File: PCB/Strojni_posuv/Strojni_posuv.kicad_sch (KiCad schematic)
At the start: 58 parts, among them J1 Conn_01x20_Pin, J15 Conn_01x06_Socket, J7 Button_maxL, J9 Button_maxR, SW1 SW_SPDT_MSM, SW2 SW_DPST_x2, SW3 SW_DPST_x2, SW4 SW_SPDT, SW5 RotaryEncoder_Switch, U1 STM32F103RBTx, Y1 16MHz

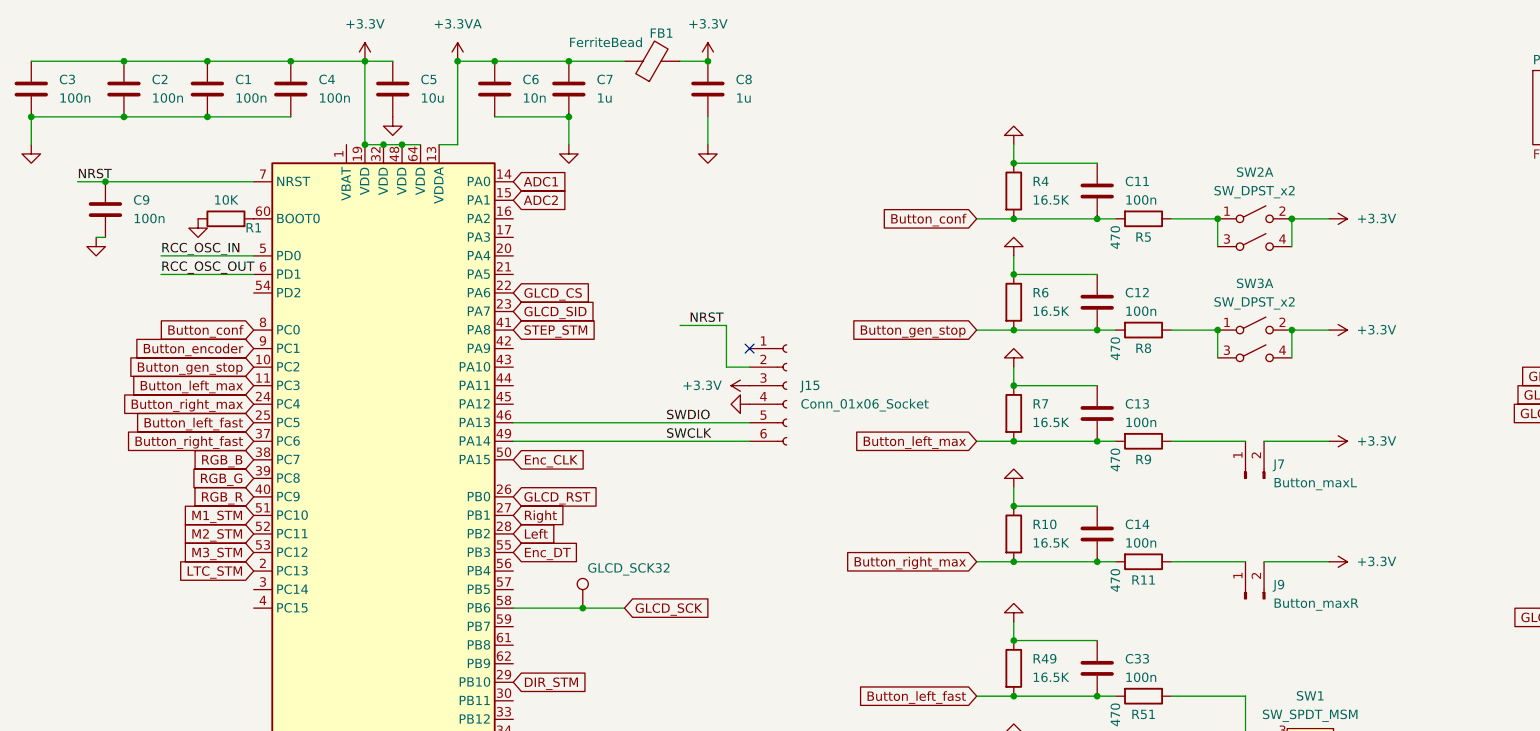
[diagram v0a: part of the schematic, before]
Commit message: Resolving problems from list
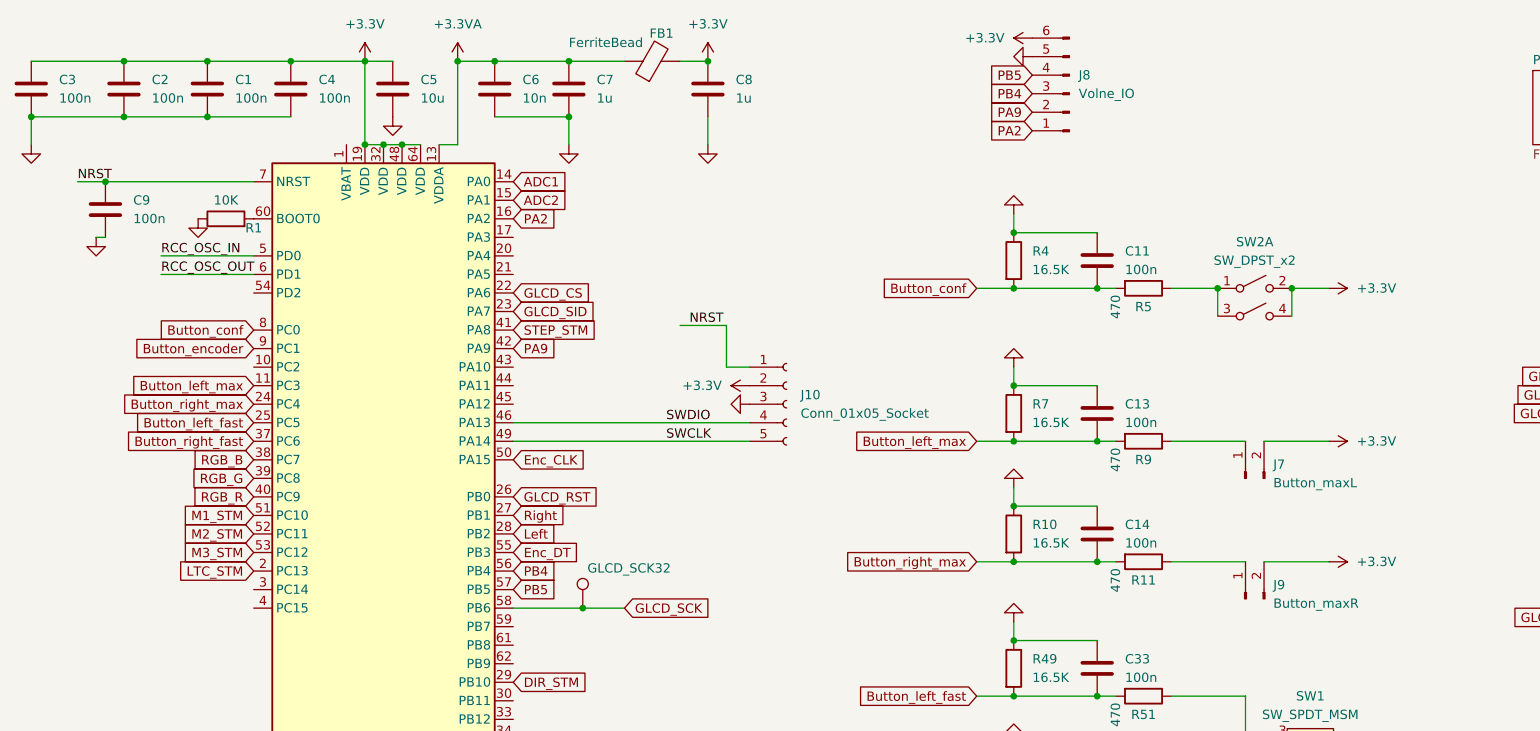
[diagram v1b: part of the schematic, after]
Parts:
- removed C12: 100n, Capacitor_SMD:C_0603_1608Metric, symbol Device:C
- removed J15: Conn_01x06_Socket, Connector_PinSocket_2.54mm:PinSocket_1x06_P2.54mm_Vertical, symbol Connector:Conn_01x06_Socket
- removed R6: 16.5K, Resistor_SMD:R_0805_2012Metric, symbol Device:R
- removed R8: 470, Resistor_SMD:R_0805_2012Metric, symbol Device:R
- removed SW3: SW_DPST_x2, Button_Switch_THT:SW_PUSH_6mm, symbol Switch:SW_DPST_x2
- added J10: Conn_01x05_Socket, Connector_JST:JST_PH_B5B-PH-K_1x05_P2.00mm_Vertical, symbol Connector:Conn_01x05_Socket
- added J8: Volne_IO, symbol Connector:Conn_01x06_Pin
- SW1: footprint Button_Switch_THT:SW_CK_JS202011CQN_DPDT_Straight -> ON_Off_ON:on_off_on
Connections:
- net +3.3V: now also J10.2 (Pin_2), J8.6 (Pin_6)
- net GND: now also J10.3 (Pin_3), J8.5 (Pin_5)
- net NRST: now also J10.1 (Pin_1)
- net SWCLK: now also J10.5 (Pin_5)
- net SWDIO: now also J10.4 (Pin_4)
- net PA2: now reaches U1.16 (PA2)
- net PA2: now also J8.1 (Pin_1)
- net PA9: now reaches U1.42 (PA9)
- net PA9: now also J8.2 (Pin_2)
- net PB4: now reaches U1.56 (PB4)
- net PB4: now also J8.3 (Pin_3)
- net PB5: now reaches U1.57 (PB5)
- net PB5: now also J8.4 (Pin_4)
- net Button_gen_stop: no longer names the net of U1.10 (PC2)
- no-connect marks 12 -> 11
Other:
- moved on the sheet: C11, R4, R5, SW2A
